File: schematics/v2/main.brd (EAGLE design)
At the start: 85.1 x 37.8 mm, 15 parts, among them IC1 MEGA8-P, Q1 BC548

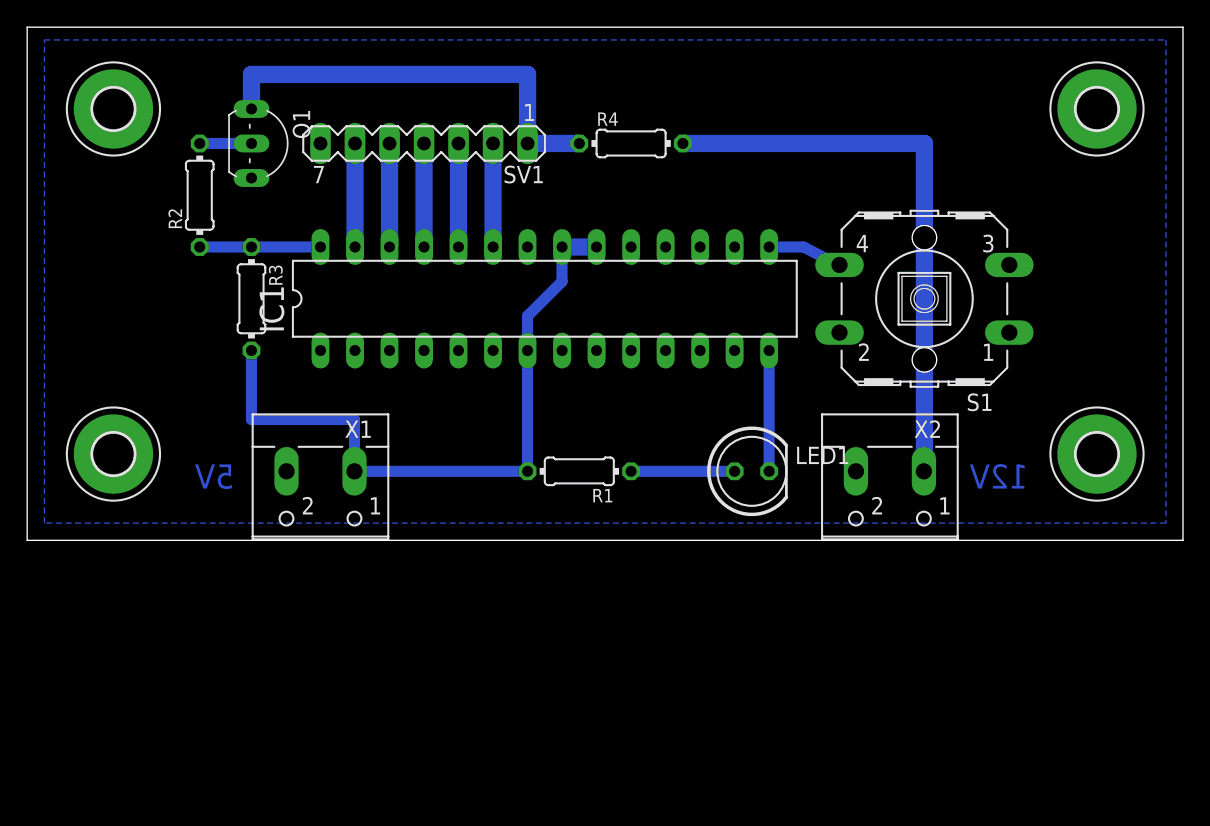
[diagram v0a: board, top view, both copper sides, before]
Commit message: Updating schematics for v2
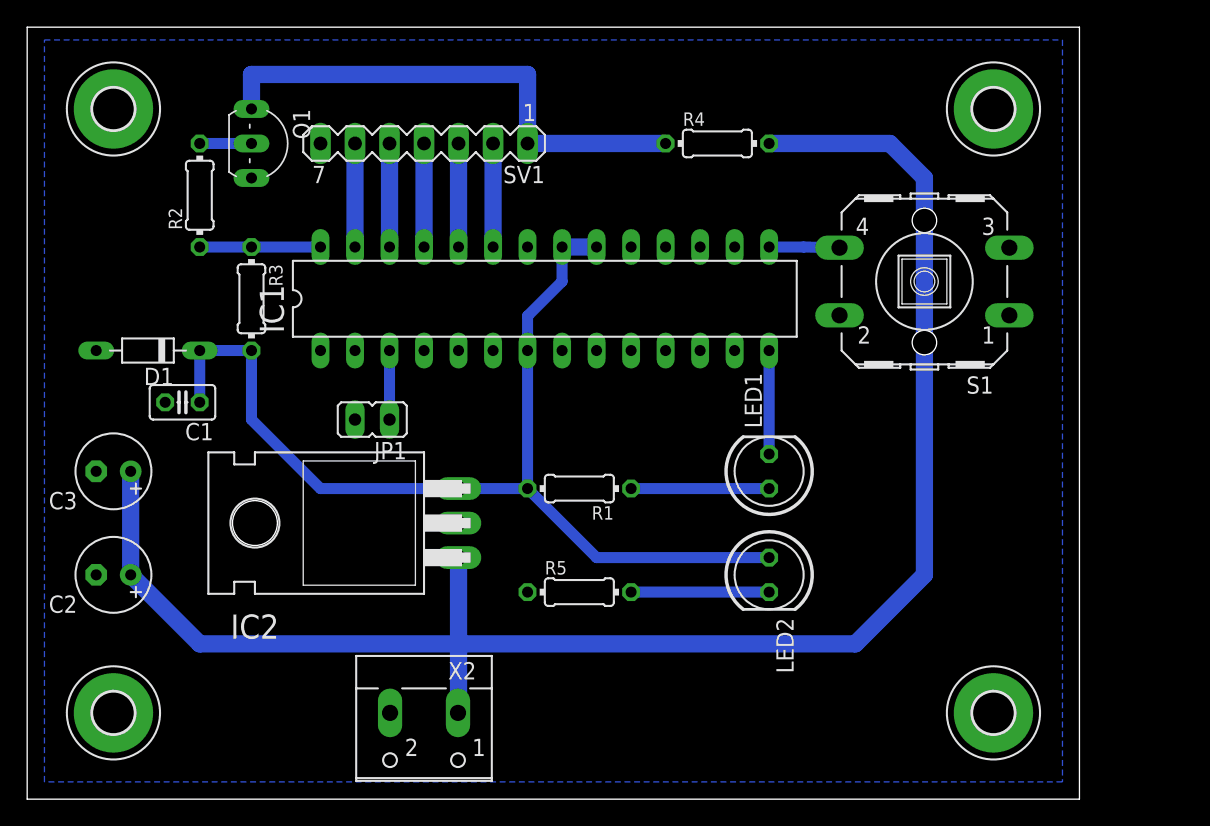
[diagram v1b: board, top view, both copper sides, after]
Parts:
- removed X1: (no value), con-wago-500:W237-102
- added C1: 100n, rcl:C025-025X050
- added C2: 47u, rcl:E2,5-6
- added C3: 10u, rcl:E2,5-6
- added D1: 1N4007, diode:D-7.5
- added IC2: 7805T, linear:TO220H
- added JP1: RS232, jumper:JP1
- added LED2: (no value), led:LED5MM
- added R5: 330, resistor:0204/7
- moved X2 38.6 mm to (41.9, 7.62)
- moved H3 20.5 mm to (83.8, 8.89)
- moved H2 19.1 mm to (19.1, 8.89)
- moved H4 7.62 mm to (83.8, 53.3)
- moved R4 6.35 mm to (63.5, 50.8)
- moved R1 1.27 mm to (53.3, 25.4)
- moved S1 1.27 mm to (78.7, 40.6)
- moved LED1 1.27 mm to (67.3, 26.7), turned to 90 degrees
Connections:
- new net N$12: LED2.K, R5.2
- new net N$13: IC1.3, JP1.1
- net +12V: now also C2.+, C3.+, IC2.1
- net +5V: now also C1.1, D1.C, IC2.3, LED2.A; no longer X1.1
- net GND: now also C1.2, C2.-, C3.-, D1.A, IC2.2, JP1.2, R5.1; no longer X1.2
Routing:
- net +12V: track 41.9 -> 123.4 mm
- net +5V: track 49.3 -> 76.4 mm
- net N$12: track 0.00 -> 10.2 mm
- net N$6: track 31.8 -> 38.1 mm
- net N$13: track 0.00 -> 5.08 mm
- net N$3: track 7.62 -> 10.2 mm
- net N$2: track 8.89 -> 7.62 mm
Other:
- board size 85.1 x 37.8 mm -> 77.5 x 56.8 mm
- board text removed: "12V"
- board text removed: "5V"
